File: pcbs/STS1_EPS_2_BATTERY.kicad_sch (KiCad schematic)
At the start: 11 parts, among them J3 Battery Pack, Q4 SI7272DP-T1-GE3, U13 TMCS1101A3B-Q1, U4 BQ29209DRBT

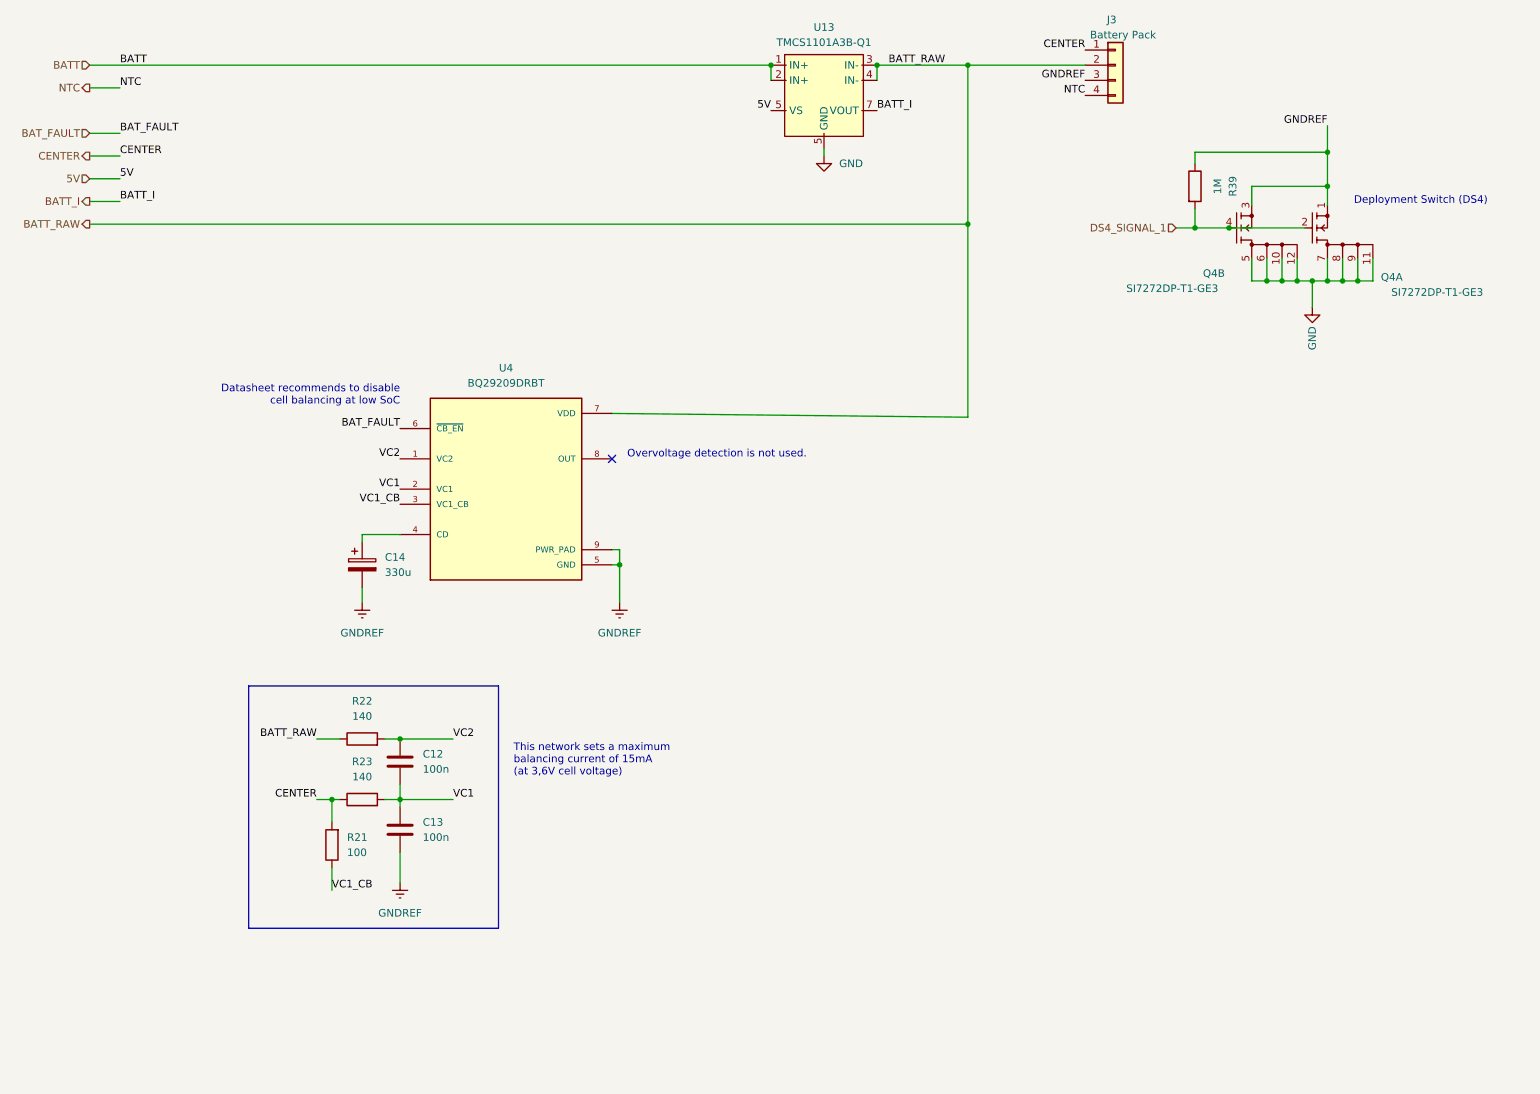
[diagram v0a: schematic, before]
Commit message: worked on sts1_eps_1
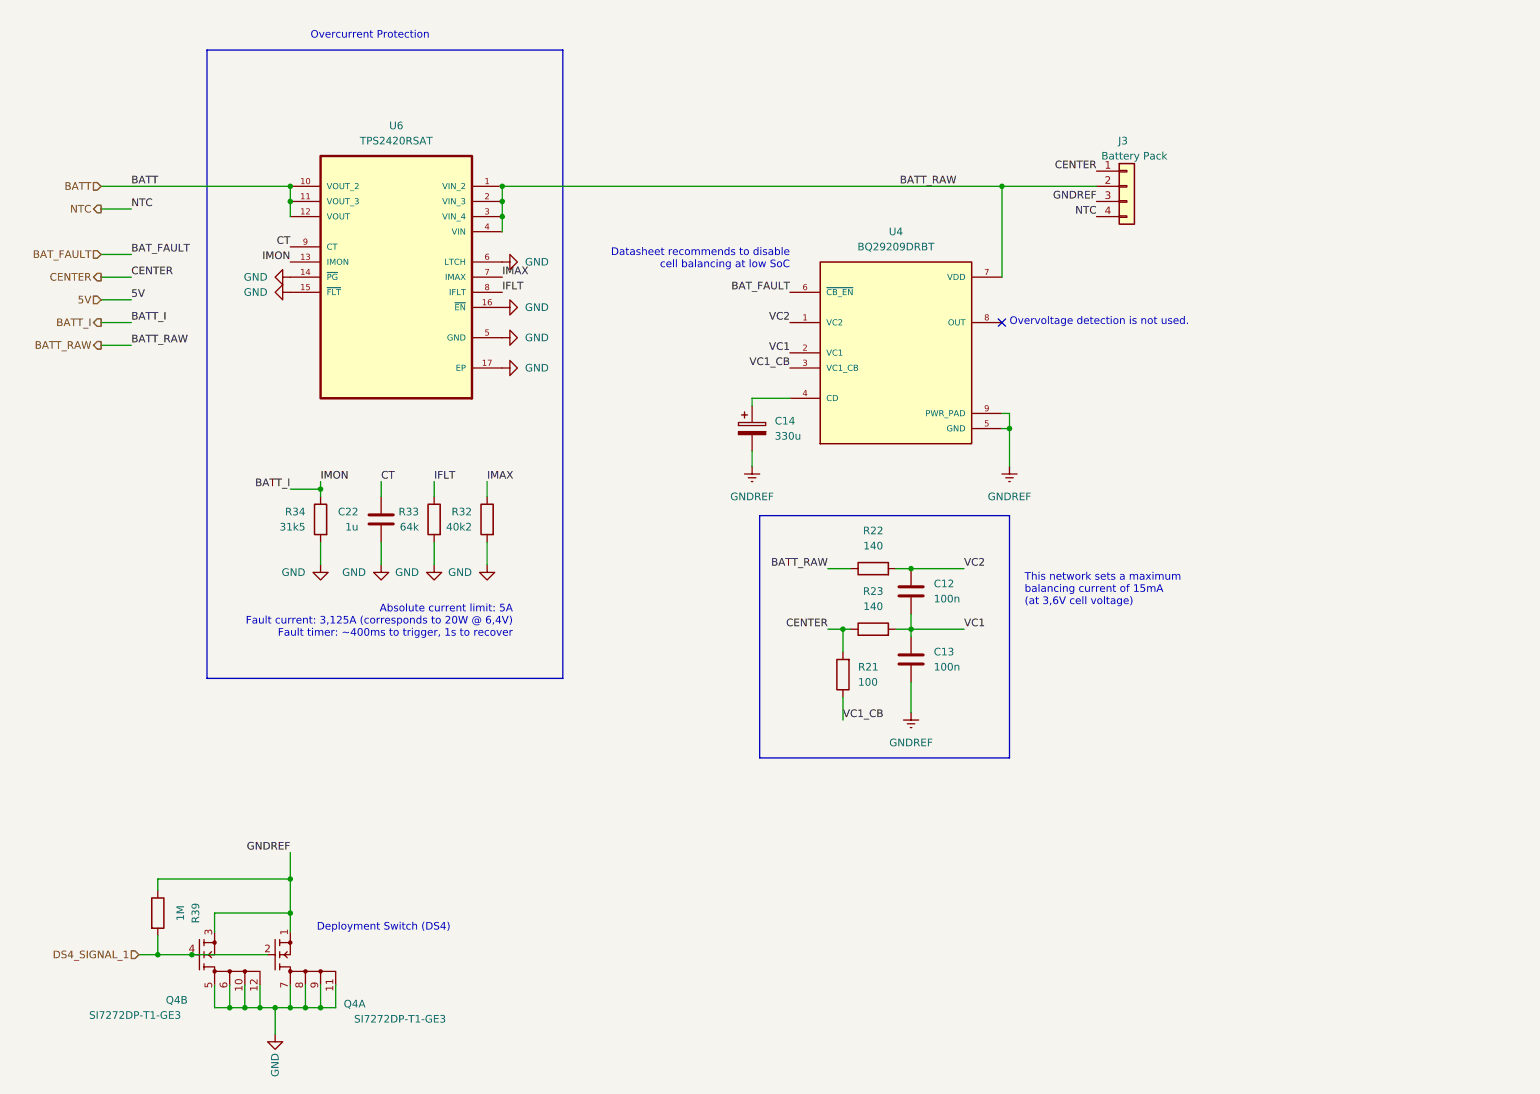
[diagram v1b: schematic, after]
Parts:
- removed U13: TMCS1101A3B-Q1, Package_SO:SOIC-8_3.9x4.9mm_P1.27mm, symbol STS_Sensor_Current:TMCS1101Q1
- added C22: 1u, Capacitor_SMD:C_0805_2012Metric, symbol Device:C
- added R32: 40k2, Resistor_SMD:R_0805_2012Metric, symbol Device:R
- added R33: 64k, Resistor_SMD:R_0805_2012Metric, symbol Device:R
- added R34: 31k5, Resistor_SMD:R_0805_2012Metric, symbol Device:R
- added U6: TPS2420RSAT, Package_DFN_QFN:VQFN-16-1EP_3x3mm_P0.5mm_EP1.45x1.45mm_ThermalVias, symbol STS_Power_Management:TPS2420RSAT
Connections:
- net BATT: now also U6.10 (VOUT_2), U6.11 (VOUT_3), U6.12 (VOUT)
- net BATT_I: now also R34.1, U6.13 (IMON)
- net BATT_RAW: now also U6.1 (VIN_2), U6.2 (VIN_3), U6.3 (VIN_4), U6.4 (VIN)
- net GND: now also C22.2, R32.2, R33.2, R34.2, U6.14 (~{PG}), U6.15 (~{FLT}), U6.16 (~{EN}), U6.17 (EP), U6.5 (GND), U6.6 (LTCH)
- new net CT: C22.1, U6.9 (CT)
- new net IFLT: R33.1, U6.8 (IFLT)
- new net IMAX: R32.1, U6.7 (IMAX)
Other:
- note added: "Absolute current limit: 5A Fault current: 3,125A (corresponds to 20W @ 6,4V) Fault timer: ~400ms to trigger, 1s to recover"
- note added: "Overcurrent Protection"
- moved on the sheet: C12, C13, C14, J3, Q4A, Q4B, R21, R22, R23, R39, U4
